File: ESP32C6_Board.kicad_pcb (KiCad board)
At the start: 4 copper layers, 100 x 50 mm, 73 parts, among them J10 JST_XH_2.54_Plug, J11 SPI_QSPI_Jumper, J16 Power_Selector_Jumper, J18 USR_BTN_EN, J19 SPI1_Headers, J2 USB_B_Micro, J3 Boot_Mode_Control_Pins, J5 3V_Selection_Header, J6 LPUART1_Headers, J7 I2C1_Headers, J8 GPIO_Headder, J9 QSPI_Header, Q1 MOSFET_SI2333DDS-T1-BE3, U1 ESP32-C6, U2 W25Q128JVSQ_SOIC208-mil, U3 USBLC6-2SC6, Y1 Crystal_ABM8W-40.0000MHZ-4-B1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, Y2 ABS07-32.768KHZ-T

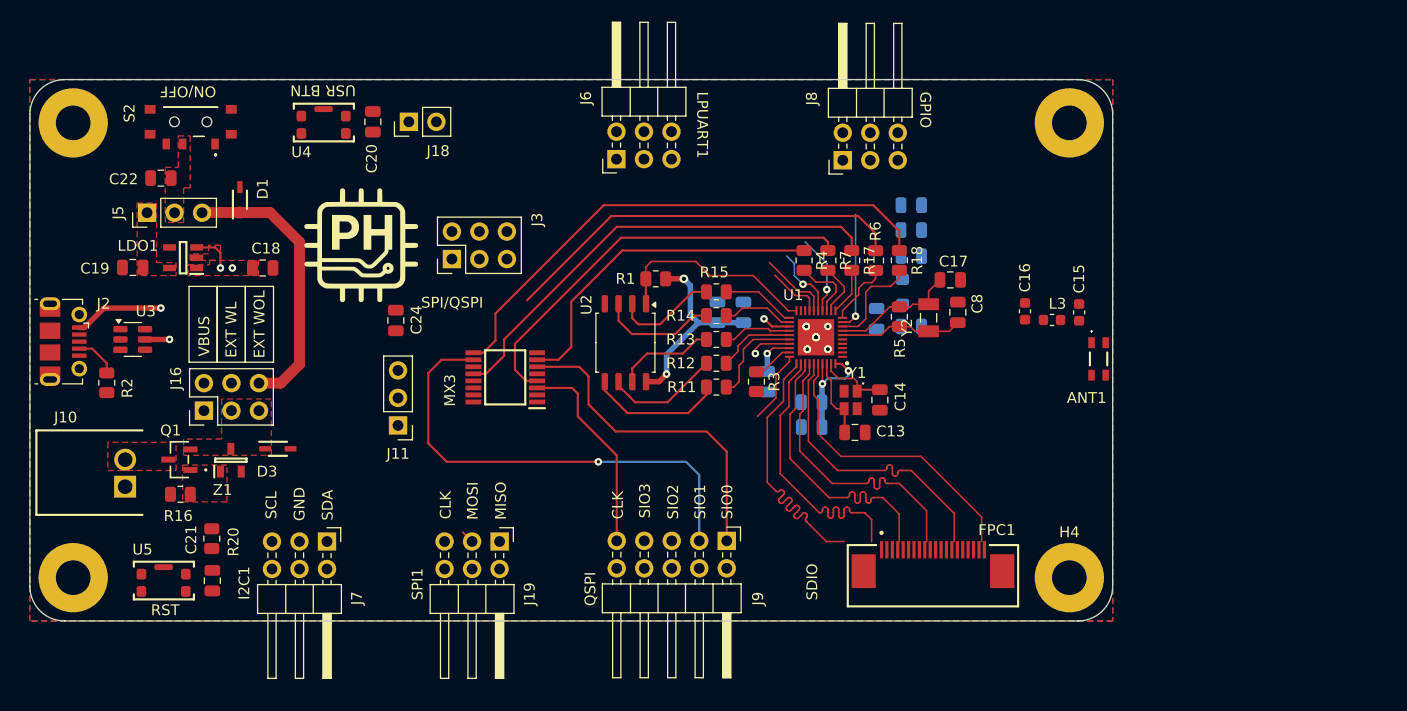
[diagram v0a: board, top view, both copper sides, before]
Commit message: Update
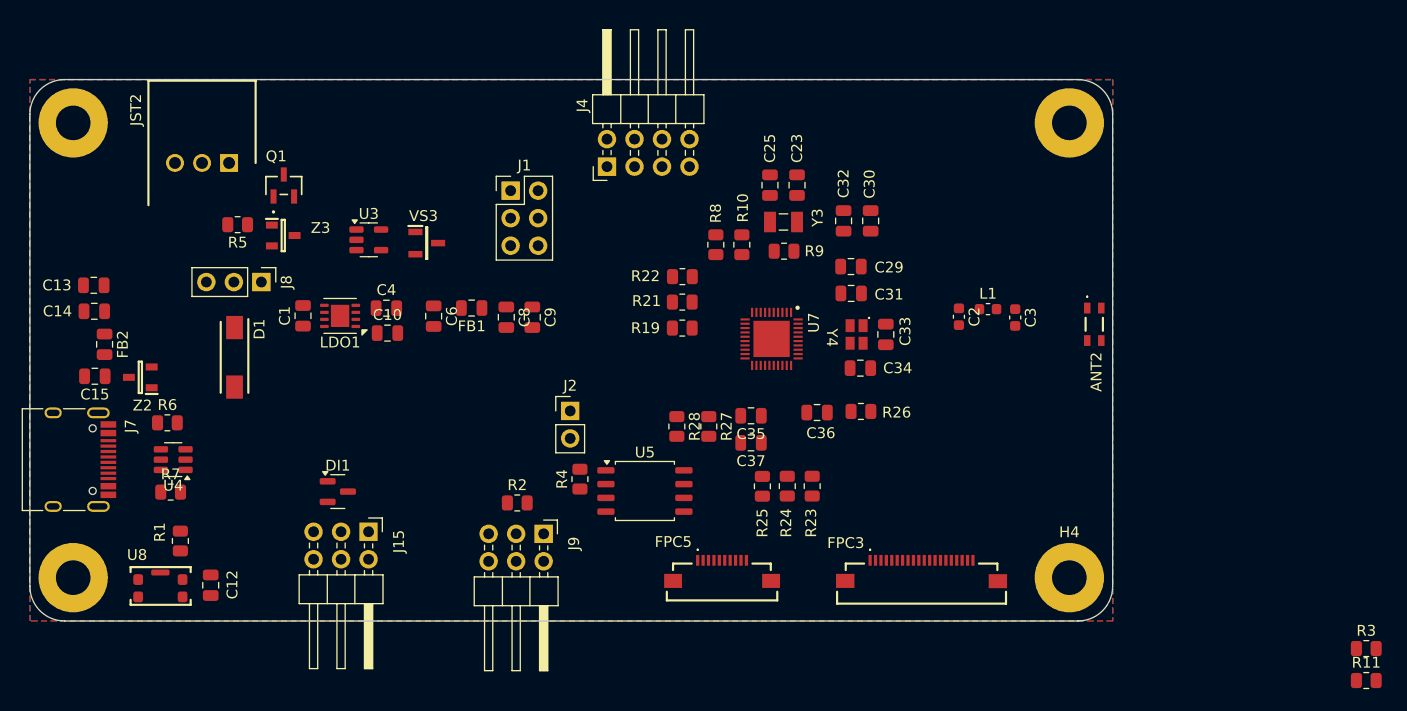
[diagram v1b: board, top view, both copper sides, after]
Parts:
- removed ANT1: Antenna_2450AT18D0100001E, Personal_Project:Antenna_2450AT18D0100001E
- removed C11, C24, C5: 100n, Capacitor_SMD:C_0805_2012Metric
- removed C16: 100n, Capacitor_SMD:C_0603_1608Metric
- removed C17: 15p, Capacitor_SMD:C_0805_2012Metric
- removed C18, C19: 1u, Capacitor_SMD:C_0805_2012Metric
- removed C20, C21: 1uF, Capacitor_SMD:C_0805_2012Metric
- removed C22: 4u7, Capacitor_SMD:C_0805_2012Metric
- removed D3: ESD_TSD05DYFR, Personal_Project:ESD_TSD05DYFR_SOD2613X100N
- removed FPC1: FPC_ZF5S-20-01-T-WT, Personal_Project:FPC_SAMTEC_ZF5S-20-01-T-WT
- removed G***: LOGO, Personal_Project:PCB_Logo
- removed J10: JST_XH_2.54_Plug, Personal_Project:Connector_Power2pin_SHDRRA2W80P0X250_1X2_740X1150X610P
- removed J11: SPI_QSPI_Jumper, Connector_PinHeader_2.54mm:PinHeader_1x03_P2.54mm_Vertical
- removed J16: Power_Selector_Jumper, Connector_PinHeader_2.54mm:PinHeader_2x03_P2.54mm_Vertical
- removed J18: USR_BTN_EN, Connector_PinHeader_2.54mm:PinHeader_1x02_P2.54mm_Vertical
- removed J19: SPI1_Headers, Connector_PinHeader_2.54mm:PinHeader_2x03_P2.54mm_Horizontal
- removed J3: Boot_Mode_Control_Pins, Connector_PinHeader_2.54mm:PinHeader_2x03_P2.54mm_Vertical
- removed J5: 3V_Selection_Header, Connector_PinHeader_2.54mm:PinHeader_1x03_P2.54mm_Vertical
- removed J6: LPUART1_Headers, Connector_PinHeader_2.54mm:PinHeader_2x03_P2.54mm_Horizontal
- removed L3: 2n, Inductor_SMD:L_0603_1608Metric
- removed MX3: MUX_SN74CB3T3257PWR, Personal_Project:MUX_SN74CB3T3257PWR_SOP65P640X120-16N
- removed R12, R13, R14, R15: 0R, Resistor_SMD:R_0805_2012Metric
- removed R16: 100k, Resistor_SMD:R_0805_2012Metric
- removed R17, R18: 33R, Resistor_SMD:R_0805_2012Metric
- removed R20: 10k, Resistor_SMD:R_0805_2012Metric
- removed S2: Switch_WS-SLSU SMT Mini Slide, Personal_Project:Switch_WS-SLSU SMT Mini Slide
- removed U1: ESP32-C6, Personal_Project:ESP32C6_QFN40P500X500X90-41N-D
- removed U2: W25Q128JVSQ_SOIC208-mil, Package_SO:SOIC-8_5.23x5.23mm_P1.27mm
- removed Y1: Crystal_ABM8W-40.0000MHZ-4-B1U-T3, Personal_Project:CRYSTAL4_ABM10W-40.0000MHZ-8-B1U-T3_ABR
- removed Y2: ABS07-32.768KHZ-T, Personal_Project:Crystal_ABS07
- removed Z1: Diode_BZX84C6V2-7-F, Personal_Project:Diode_BZX84C6V2_SOT96P240X110-3N
- added ANT2: Antenna_2450AT18D0100001E, Personal_Project:Antenna_2450AT18D0100001E, F.Cu at (178.3, 92.6)
- added C23: 15p, Capacitor_SMD:C_0805_2012Metric, F.Cu at (150.8, 79.8)
- added C25: 15p, Capacitor_SMD:C_0805_2012Metric, F.Cu at (148.3, 79.8)
- added C29: 1u, Capacitor_SMD:C_0805_2012Metric, F.Cu at (155.8, 87.3)
- added C30: 100n, Capacitor_SMD:C_0805_2012Metric, F.Cu at (157.7, 83.0)
- added C31: 10n, Capacitor_SMD:C_0805_2012Metric, F.Cu at (155.8, 89.8)
- added C32: 100n, Capacitor_SMD:C_0805_2012Metric, F.Cu at (155.2, 83.0)
- added C33: 2p, Capacitor_SMD:C_0805_2012Metric, F.Cu at (159.1, 93.5)
- added C34: 2p, Capacitor_SMD:C_0805_2012Metric, F.Cu at (156.7, 96.7)
- added C35: 100n, Capacitor_SMD:C_0805_2012Metric, F.Cu at (146.6, 101.0)
- added C36: 100n, Capacitor_SMD:C_0805_2012Metric, F.Cu at (152.7, 100.8)
- added C37: 1u, Capacitor_SMD:C_0805_2012Metric, F.Cu at (146.6, 103.5)
- added DI1: Diode_PESD5V0U2BT-Q, Package_TO_SOT_SMD:SOT-23, F.Cu at (108.4, 108.0)
- added FB1: BLM21AG121BH1D, Capacitor_SMD:C_0805_2012Metric, F.Cu at (120.8, 91.1)
- added FB2: Part # MI0805K601R-10, Capacitor_SMD:C_0805_2012Metric, F.Cu at (86.9, 94.5)
- added FPC3: FPC_0545482072, Personal_Project:FPC_0545482072, F.Cu at (162.3, 116.0)
- added FPC5: FPC_0545481072, Personal_Project:FPC_0545481072, F.Cu at (143.9, 116.0)
- added J1: Boot_Mode_Control_Pins, Connector_PinHeader_2.54mm:PinHeader_2x03_P2.54mm_Vertical, F.Cu at (124.4, 80.3)
- added J15: I2C1_Headers, Personal_Project:PinHeader_2x03_P2.54mm_Horizontal_Court, F.Cu at (111.3, 111.8)
- added J4: I/O_HDR, Connector_PinHeader_2.54mm:PinHeader_2x04_P2.54mm_Horizontal, F.Cu at (133.3, 78.0)
- added JST2: JST_S3B-XH-2.54, Personal_Project:JST_S3B-XH-SHDRRA3W64P0X250_1X3_990X1150X610P, F.Cu at (98.4, 77.7)
- added R10: 33R, Resistor_SMD:R_0805_2012Metric, F.Cu at (145.8, 85.2)
- added R19: 33R, Resistor_SMD:R_0805_2012Metric, F.Cu at (140.2, 93.0)
- added R21: 33R, Resistor_SMD:R_0805_2012Metric, F.Cu at (140.2, 90.5)
- added R22: 33R, Resistor_SMD:R_0805_2012Metric, F.Cu at (140.3, 88.2)
- added R23: 0R, Resistor_SMD:R_0805_2012Metric, F.Cu at (152.2, 107.5)
- added R24: 0R, Resistor_SMD:R_0805_2012Metric, F.Cu at (149.9, 107.5)
- added R25: 0R, Resistor_SMD:R_0805_2012Metric, F.Cu at (147.7, 107.6)
- added R26: 100k, Resistor_SMD:R_0805_2012Metric, F.Cu at (156.8, 100.7)
- added R27: 0R, Resistor_SMD:R_0805_2012Metric, F.Cu at (142.7, 102.0)
- added R28: 0R, Resistor_SMD:R_0805_2012Metric, F.Cu at (139.8, 102.0)
- added R8: 33R, Resistor_SMD:R_0805_2012Metric, F.Cu at (143.3, 85.2)
- added R9: 0R, Resistor_SMD:R_0805_2012Metric, F.Cu at (149.7, 85.8)
- added U7: ESP32-C6, Personal_Project:ESP32C6_QFN40P500X500X90-41N-D, F.Cu at (148.5, 94.0)
- added U8: ~, Personal_Project:Button_KMR231GLFS, F.Cu at (89.5, 118.3)
- added VS3: VS_STM1818TWX7F, Personal_Project:SOT-23-3_SOT103P237X112-3N, F.Cu at (116.7, 85.1)
- added Y3: ABS07-32.768KHZ-T, Personal_Project:Crystal_ABS07, F.Cu at (149.6, 83.2)
- added Y4: Crystal_ABM8W-40.0000MHZ-4-B1U-T3, Personal_Project:CRYSTAL4_ABM10W-40.0000MHZ-8-B1U-T3_ABR, F.Cu at (156.3, 93.5)
- added Z2: Diode_BZX84C6V2-7-F, Personal_Project:Diode_BZX84C6V2_SOT96P240X110-3N, F.Cu at (90.2, 97.5)
- added Z3: Diode_BZX84C6V2-7-F, Personal_Project:Diode_BZX84C6V2_SOT96P240X110-3N, F.Cu at (103.4, 84.4)
- C1, C6: moved to F.Cu
- C10: value 100n -> 2u2; moved to F.Cu
- C12: value 100n -> 1uF; moved to F.Cu
- C13: value 2p -> 100n
- C14: value 2p -> 4u7
- C15: footprint Capacitor_SMD:C_0603_1608Metric -> Capacitor_SMD:C_0805_2012Metric
- C2: value 10n -> 100n; footprint Capacitor_SMD:C_0805_2012Metric -> Capacitor_SMD:C_0603_1608Metric; moved to F.Cu
- C3: value 10u -> 100n; footprint Capacitor_SMD:C_0805_2012Metric -> Capacitor_SMD:C_0603_1608Metric; moved to F.Cu
- C4: value 1u -> 10n; moved to F.Cu
- C8: value 15p -> 1u
- C9: value 1u -> 100n; moved to F.Cu
- D1: value ESD_TSD03DYFR -> SMAJ6.0A; footprint Personal_Project:ESD_TSD05DYFR_SOD2613X100N -> Personal_Project:DO-214AC-2
- J2: value USB_B_Micro -> USR_BTN_EN; footprint Connector_USB:USB_Micro-B_Molex-105017-0001 -> Connector_PinHeader_2.54mm:PinHeader_1x02_P2.54mm_Vertical
- J7: value I2C1_Headers -> USB_C_Receptacle_USB2.0_16P; footprint Connector_PinHeader_2.54mm:PinHeader_2x03_P2.54mm_Horizontal -> Connector_USB:USB_C_Receptacle_HRO_TYPE-C-31-M-12
- J8: value GPIO_Headder -> PWR_SRC_JMP; footprint Connector_PinHeader_2.54mm:PinHeader_2x03_P2.54mm_Horizontal -> Connector_PinHeader_2.54mm:PinHeader_1x03_P2.54mm_Vertical
- J9: value QSPI_Header -> UART1_HDR; footprint Connector_PinHeader_2.54mm:PinHeader_2x05_P2.54mm_Horizontal -> Personal_Project:PinHeader_2x03_P2.54mm_Horizontal_Court
- L1: footprint Inductor_SMD:L_0805_2012Metric_Pad1.05x1.20mm_HandSolder -> Inductor_SMD:L_0603_1608Metric; moved to F.Cu
- LDO1: value LDO_TLV75733PDBVR -> LDO_LDLN050PU33R; footprint Personal_Project:LDO_SOT95P280X145-5N -> Package_DFN_QFN:DFN-8-1EP_3x3mm_P0.65mm_EP1.7x2.05mm
- R1, R3: value 100k -> 10k
- R11: value 0R -> 10k
- R2: value 100k -> 33R
- R4: value 33R -> 100k
- R5: value 0R -> 100k
- R6, R7: value 33R -> 5k1
- U3: value USBLC6-2SC6 -> SN74LVC1G07DBVR; footprint Package_TO_SOT_SMD:SOT-23-6 -> Package_TO_SOT_SMD:SOT-23-5
- U4: value ~ -> USBLC6-2SC6; footprint Personal_Project:Button_KMR231GLFS -> Package_TO_SOT_SMD:SOT-23-6
- U5: value ~ -> W25Q128JVSQ_SOIC208-mil; footprint Personal_Project:Button_KMR231GLFS -> Package_SO:SOIC-8_5.23x5.23mm_P1.27mm
- moved C15 91.1 mm to (86.0, 97.4), turned to 180 degrees
- moved C14 73.0 mm to (86.0, 91.4), turned to 180 degrees
- moved C13 71.6 mm to (85.9, 89.0), turned to 180 degrees
- moved R6 67.1 mm to (92.7, 101.7), turned to 0 degrees
- moved R11 65.9 mm to (203.4, 125.5), turned to 0 degrees
- moved R7 64.4 mm to (93.0, 108.1), turned to 0 degrees
- moved R5 61.7 mm to (99.2, 83.4), turned to 180 degrees
- moved R3 61.5 mm to (203.4, 122.5), turned to 0 degrees
- moved J8 54.9 mm to (101.4, 88.7), turned to -90 degrees
- moved C12 54.7 mm to (96.7, 116.7), turned to 90 degrees
- moved R1 50.1 mm to (93.9, 112.6), turned to 90 degrees
- moved C4 49.0 mm to (112.9, 91.1)
- moved C1 48.1 mm to (105.2, 91.8), turned to 90 degrees
- moved U5 48.0 mm to (136.8, 108.0)
- moved J2 47.2 mm to (129.9, 100.6), turned to 0 degrees
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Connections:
- C1 pad 1: +3.3V -> /Power_Management/PWR+_PS
- C12 pad 1: +3.3V -> GND
- C12 pad 2: GND -> /Interfaces/USR_BTN_P
- C13 pad 1: Net-(U1-XTAL_N) -> USB_VBUS+
- C14 pad 1: Net-(U1-XTAL_P) -> USB_VBUS+
- C15 pad 1: /RF_ANT -> USB_VBUS+
- C2 pad 1: +3.3V -> /ESP32-C6/RF_LNA_IN
- C3 pad 1: +3.3V -> /RF_USB_Memory/RF_ANT
- C4 pad 1: +3.3V -> Net-(LDO1-FB)
- C6 pad 1: Net-(U1-VDDA3P3_1) -> +3.3V
- C8 pad 1: Net-(U1-XTAL_32K_P) -> +3.3VA
- C9 pad 1: /VDD_SPI -> +3.3VA
- D1 pad 1: /EXT_POWER+_NOLDO -> /Power_Management/PWR+_PS
- J2 pad 1: +5V_VBUS -> /ESP32-C6/GPIO3_USR_BTN
- J2 pad 2: /USB_D2- -> /Interfaces/USR_BTN_P
- J8 pad 1: /GPIO3_USR_BTN -> /Power_Management/PWR+_PP
- J8 pad 2: GND -> /Power_Management/PWR+_PS
- J8 pad 3: GND -> USB_VBUS+
- J9 pad 1: /GPIO7_FSPID_MOSI/SIO0_1 -> GND
- J9 pad 3: /GPIO2_FSPIQ_MISO/SIO1_1 -> Net-(J9-Pin_3)
- J9 pad 5: /GPIO5_FSPIWP_SIO2_1 -> GND
- L1 pad 1: +3.3V -> /RF_USB_Memory/RF_ANT
- L1 pad 2: Net-(U1-VDDA3P3_1) -> /ESP32-C6/RF_LNA_IN
- LDO1 pad 1: /LDO_IN -> +3.3V
- LDO1 pad 2: GND -> unconnected-(LDO1-NC-Pad2)
- LDO1 pad 3: /LDO_IN -> Net-(LDO1-FB)
- LDO1 pad 4: unconnected-(LDO1-NC-Pad4) -> GND
- LDO1 pad 5: /LD_OUT_3V3 -> /Power_Management/PWR+_PS
- Q1 pad 1: /MOSFET_GATE -> /Power_Management/PWR+_GATE
- Q1 pad 2: /EXT_POWER+_PP -> /Power_Management/PWR+_PP
- Q1 pad 3: /EXT_POWER+ -> /Power_Management/PWR+
- R1 pad 1: /VDD_SPI -> /Interfaces/USR_BTN_P
- R1 pad 2: /SPICS0_Chip_Select -> +3.3V
- R11 pad 1: /SPID_Data_In_R -> +3.3V
- R11 pad 2: /SPID_Data_In -> /ESP32-C6/GPIO10_I2C_SCL
- R2 pad 1: GND -> /ESP32-C6/GPIO17_U0TXD
- R2 pad 2: Net-(J2-ID) -> Net-(J9-Pin_3)
- R3 pad 1: /U0TXD_R -> +3.3V
- R3 pad 2: /GPIO17_U0TXD -> /ESP32-C6/GPIO11_I2C_SDA
- R4 pad 1: /GPIO7_FSPID_MOSI/SIO0_R -> +3.3V_VDD_SPI
- R4 pad 2: /GPIO7_FSPID_MOSI/SIO0 -> /ESP32-C6/SPICS0_Chip_Select
- R5 pad 1: Net-(U1-XTAL_32K_N) -> /Power_Management/PWR+_GATE
- R5 pad 2: Net-(U1-XTAL_32K_P) -> GND
- R6 pad 1: /GPIO4_FSPIHD_SIO3 -> Net-(J7-CC1)
- R6 pad 2: /GPIO4_FSPIHD_SIO3_R -> GND
- R7 pad 1: /GPIO6_FSPICLK_R -> Net-(J7-CC2)
- R7 pad 2: /GPIO6_FSPICLK -> GND
- U3 pad 1: /USB_D2- -> unconnected-(U3-NC-Pad1)
- U3 pad 2: GND -> /Power_Management/RST_PWR
- U3 pad 3: /USB_D2+ -> GND
- U3 pad 4: /USB_D+ -> /ESP32-C6/RST_CHIP_PU_D
- U3 pad 5: +5V_VBUS -> +3.3V
- U4 pad 1: /GPIO3_USR_BTN_E -> /ESP32-C6/USB_D-
- U4 pad 2: /GPIO3_USR_BTN_E -> GND
- U4 pad 3: GND -> /ESP32-C6/USB_D+
- U4 pad 4: GND -> /RF_USB_Memory/USB_D2+
- U4 pad 5: GND -> USB_VBUS+
- U5 pad 1: /CHIP_PU_D -> /ESP32-C6/SPICS0_Chip_Select
- U5 pad 2: /CHIP_PU_D -> /ESP32-C6/SPIQ_Data_Out
- U5 pad 3: GND -> /ESP32-C6/SPIWP_Write_Protect
- U5 pad 5: GND -> /ESP32-C6/SPID_Data_In
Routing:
- net /GPIO2_FSPIQ_MISO/SIO1_R: track 49.2 -> 0.00 mm
- net /GPIO2_FSPIQ_MISO/SIO1_1: track 43.5 -> 0.00 mm, vias 1 -> 0
- net /GPIO5_FSPIWP_SIO2_R: track 43.0 -> 0.00 mm
- net /GPIO6_FSPICLK_R: track 38.8 -> 0.00 mm
- net /GPIO4_FSPIHD_SIO3_R: track 37.7 -> 0.00 mm
- net /GPIO7_FSPID_MOSI/SIO0_R: track 31.3 -> 0.00 mm
- net /GPIO7_FSPID_MOSI/SIO0_1: track 30.5 -> 0.00 mm
- net /GPIO22_SDIO_DATA2: track 27.6 -> 0.00 mm
- net /GPIO21_SDIO_DATA1: track 27.5 -> 0.00 mm
- net /GPIO23_SDIO_DATA3: track 27.3 -> 0.00 mm
- net /GPIO20_SDIO_DATA0: track 27.1 -> 0.00 mm
- net /GPIO19_SDIO_CLK: track 27.0 -> 0.00 mm
- net /GPIO18_SDIO_CMD: track 26.9 -> 0.00 mm
- net /EXT_POWER+_NOLDO: track 25.9 -> 0.00 mm
- net +5V_VBUS: track 22.8 -> 0.00 mm, vias 2 -> 0
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- removed copper zone on F.Cu, net /EXT_POWER+
- removed copper zone on F.Cu, net /EXT_POWER+_PP
- removed copper zone on F.Cu, net /LDO_IN
- removed copper zone on In2.Cu, net /LDO_IN
- removed copper zone on F.Cu, net /LD_OUT_3V3
- removed copper zone on F.Cu, net /MOSFET_GATE
- removed copper zone on F.Cu, net /POWER_3V3
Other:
- board text removed: "CLK"
- board text removed: "EXT WL"
- board text removed: "EXT WOL"
- board text removed: "GND"
- board text removed: "GPIO"
- board text removed: "I2C1"
- board text removed: "LPUART1"
- board text removed: "MISO"
- board text removed: "MOSI"
- board text removed: "ON/OFF"
- board text removed: "QSPI"
- board text removed: "RST"
- board text removed: "SCL"
- board text removed: "SDA"
- board text removed: "SDIO"
- board text removed: "SIO0"
- board text removed: "SIO1"
- board text removed: "SIO2"
- board text removed: "SIO3"
- board text removed: "SPI/QSPI"
- board text removed: "SPI1"
- board text removed: "USR BTN"
- board text removed: "VBUS"
